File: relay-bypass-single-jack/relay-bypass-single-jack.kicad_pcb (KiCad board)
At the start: 2 copper layers, 57 x 37 mm, 64 parts, among them J1 3, J2 TC2030, J3 AudioJack3_Switch, J4 AudioJack3_Switch, J5 Conn_Coaxial_Small, K1 IM05JR, Q1 DMP3099L, Q2 DMN62D0U-7, Q3 DMN62D0U-7, U1 TLV76701DRVR, U2 STM32C011F4Ux, U3 TLP170AM

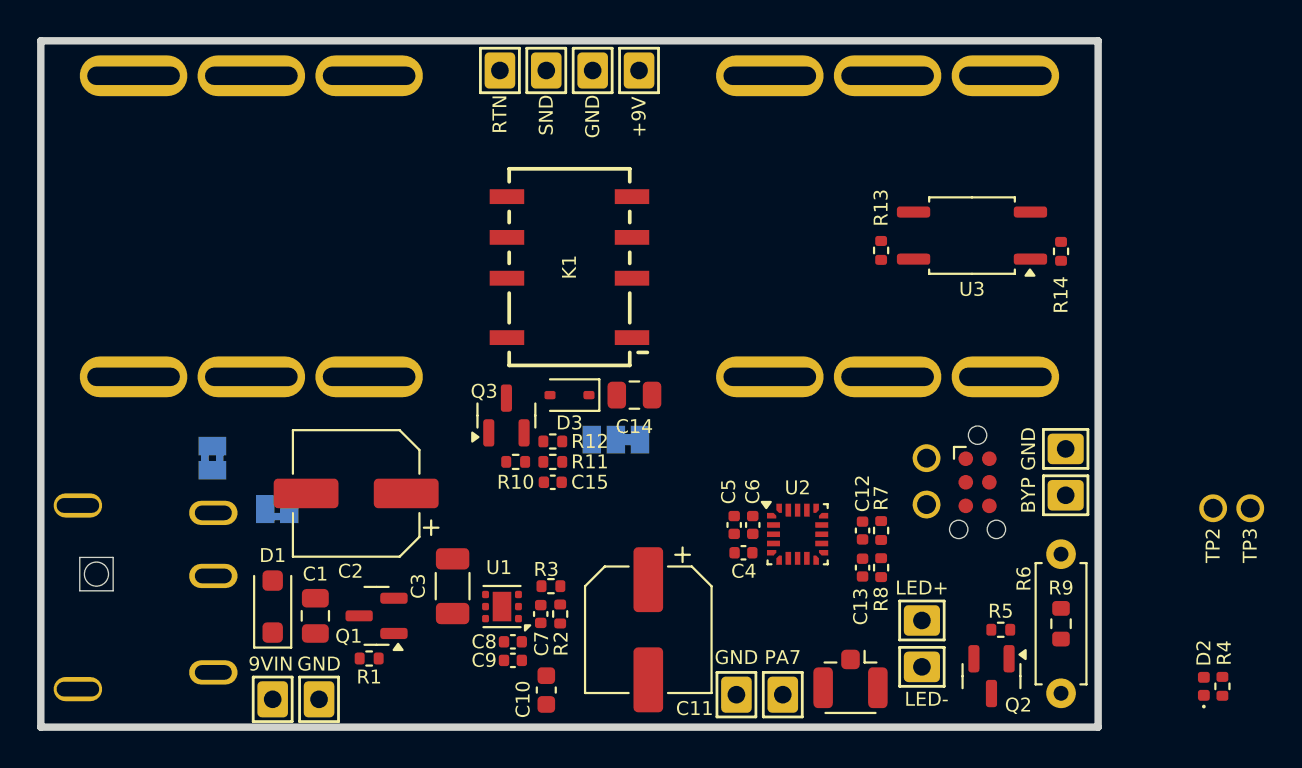
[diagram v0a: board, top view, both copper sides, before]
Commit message: Scratchwork
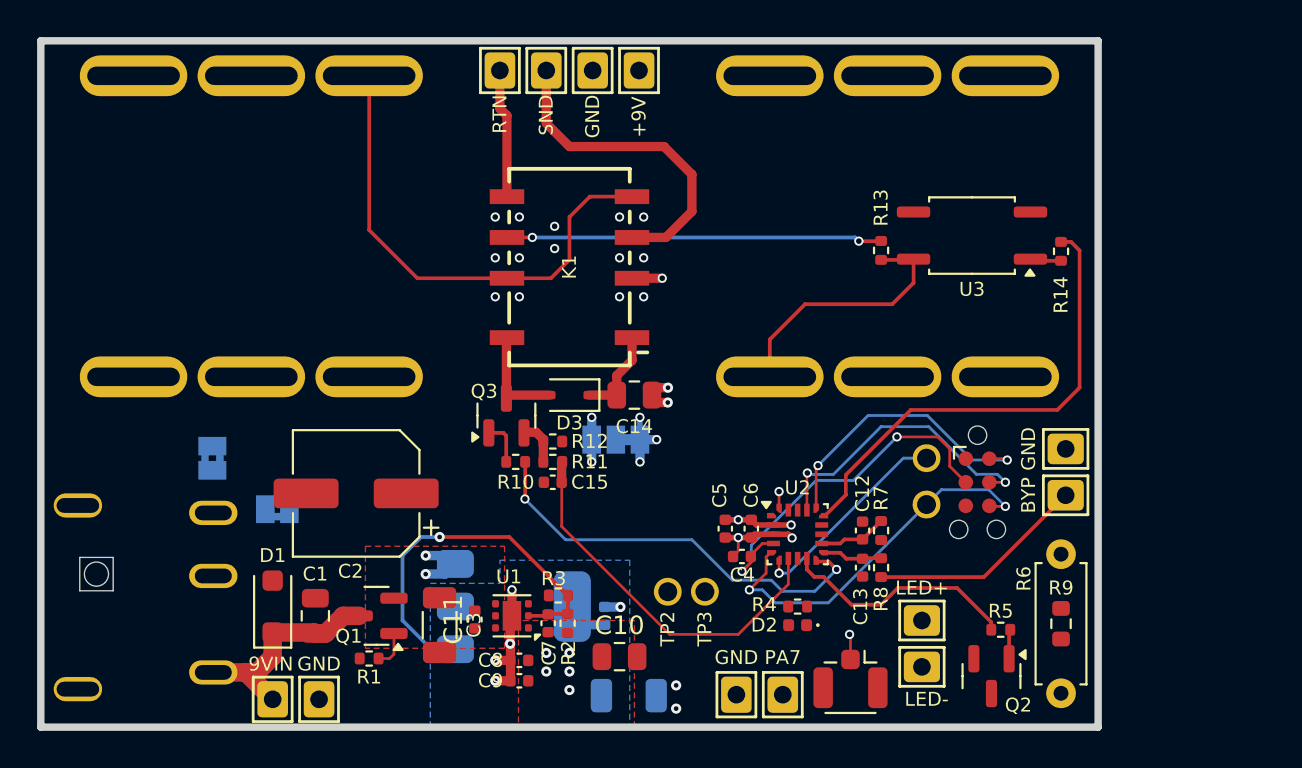
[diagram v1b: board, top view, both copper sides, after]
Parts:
- removed REF**: Footswitch_SPST, g-art:Footswitch_SPST
- added C16: 4.7u, Capacitor_SMD:C_1206_3216Metric, B.Cu at (72.8, 156.3)
- added C17: 100n, Capacitor_SMD:C_0402_1005Metric, B.Cu at (71.5, 152.0)
- added U4: LM317LCPK, Package_TO_SOT_SMD:SOT-223, B.Cu at (66.5, 151.5)
- C10: footprint Capacitor_SMD:C_0603_1608Metric -> Capacitor_SMD:C_0805_2012Metric
- C11: value 47u -> 100n; footprint Capacitor_SMD:CP_Elec_6.3x5.8 -> Capacitor_SMD:C_0402_1005Metric
- moved TP2 29.7 mm to (74.8, 150.7)
- moved TP3 29.7 mm to (76.8, 150.7)
- moved R4 23.3 mm to (81.8, 151.5), turned to 180 degrees
- moved D2 22.1 mm to (81.8, 152.5), turned to 180 degrees
- moved C11 9.37 mm to (64.5, 152.2), turned to 90 degrees
- moved C10 4.34 mm to (72.2, 154.2), turned to 0 degrees
- moved C3 2.21 mm to (62.5, 152.5), turned to -90 degrees
- moved C9 1.15 mm to (66.8, 155.5)
- moved C8 1.06 mm to (66.8, 154.4)
- moved U1 0.73 mm to (66.5, 152.0)
- moved C7 0.64 mm to (68.4, 152.4)
- moved R2 0.64 mm to (69.5, 152.4)
- moved R3 0.64 mm to (69.0, 150.9)
- moved C5 0.52 mm to (78.0, 147.3)
- moved C4 0.22 mm to (78.8, 148.8)
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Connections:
- C11 pad 1: +3.3V -> +9V
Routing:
- net /Relay_And_Jacks/IN: track 0.00 -> 26.7 mm
- net /MUTE: track 0.00 -> 25.8 mm
- net /RLY_SET: track 0.00 -> 22.6 mm, vias 0 -> 2
- net /FB: track 0.00 -> 20.8 mm, vias 0 -> 1
- net /ISNS: track 0.00 -> 20.6 mm
- net /UART1_TX: track 0.00 -> 20.3 mm, vias 0 -> 2
- net /Relay_And_Jacks/OUT_R: track 0.00 -> 20.3 mm, vias 0 -> 2
- net /NRST: track 0.00 -> 19.7 mm, vias 0 -> 2
- net /Relay_And_Jacks/SEND: track 0.00 -> 17.6 mm
- net /SWCLK: track 0.00 -> 15.9 mm, vias 0 -> 2
- net /SWDIO: track 0.00 -> 15.6 mm, vias 0 -> 2
- net /Relay_And_Jacks/OUT: track 0.00 -> 14.1 mm
- net GNDD: track 0.00 -> 14.0 mm, vias 0 -> 9
- net /LED_EXT: track 0.00 -> 12.9 mm
- net +9VIN: track 0.00 -> 12.0 mm
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- added copper zone on B.Cu, net +3.3V
- added copper zone on F.Cu, net +3.3V
- added copper zone on In2.Cu, net +3.3V
- added copper zone on F.Cu, net +9V
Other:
- copper layers 2 -> 4
